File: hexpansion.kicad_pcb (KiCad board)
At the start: 2 copper layers, 32 x 36.6 mm, 7 parts, among them J1 Hexpansion-Connector, J2 Conn_02x10_Odd_Even

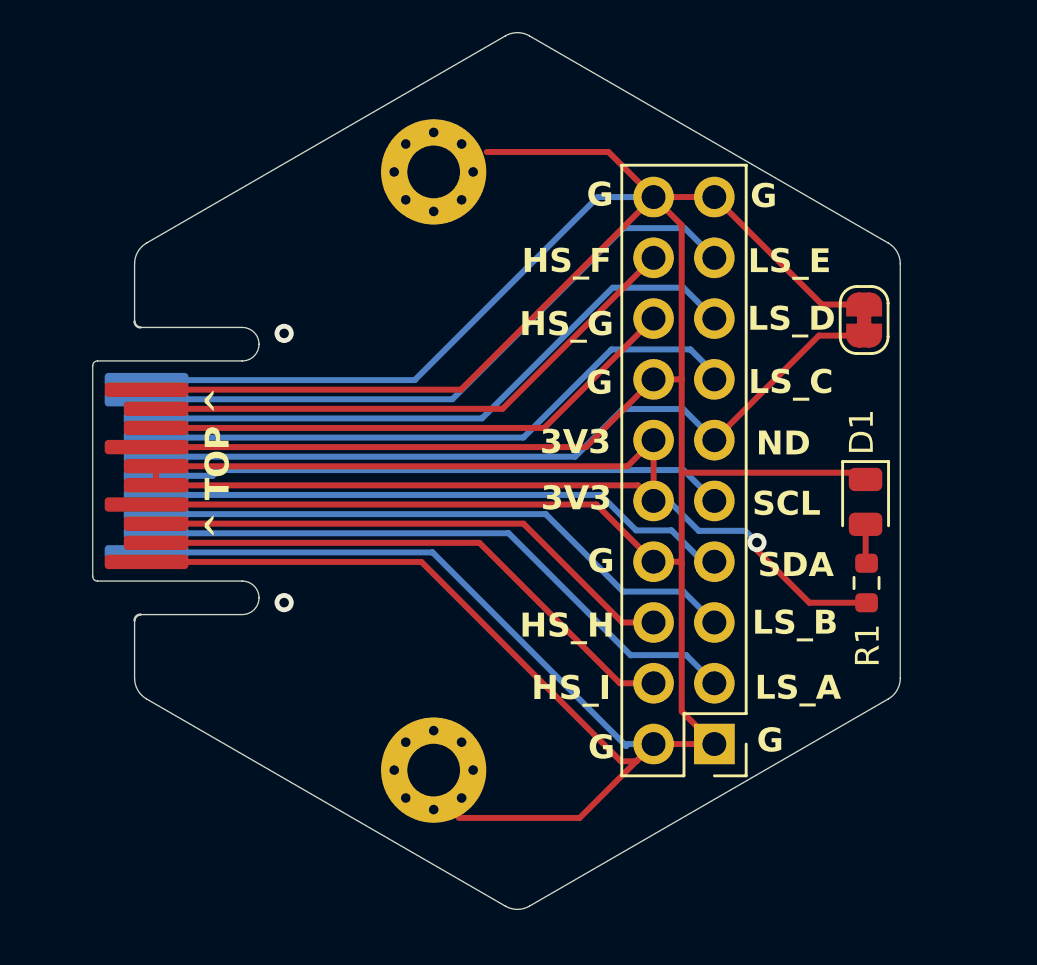
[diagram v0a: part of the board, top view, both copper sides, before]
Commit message: rough place of pcb
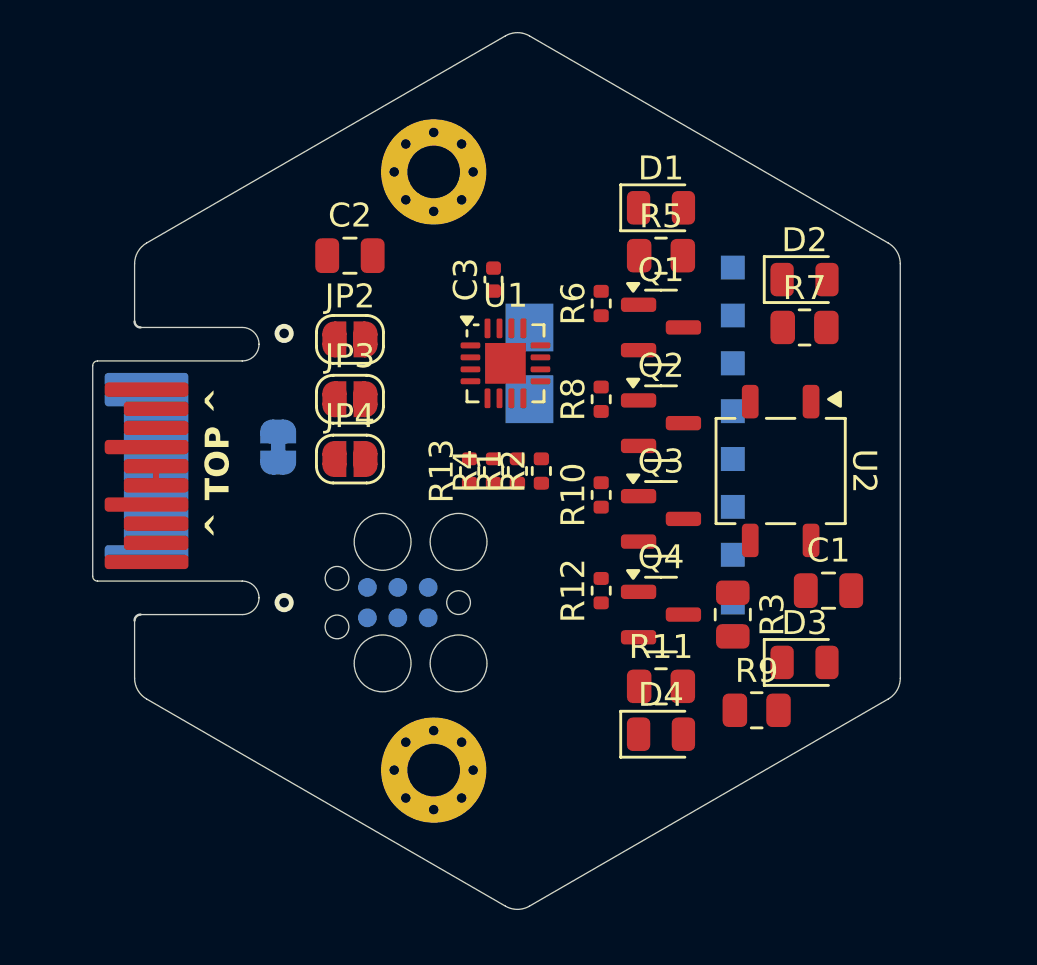
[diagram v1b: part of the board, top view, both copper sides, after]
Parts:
- added C1: 4.7 uF, Capacitor_SMD:C_0805_2012Metric, F.Cu at (129.0, 105.0)
- added C2: 4.7 uF, Capacitor_SMD:C_0805_2012Metric, F.Cu at (109.0, 91.0)
- added C3: 0.1 uF, Capacitor_SMD:C_0402_1005Metric, F.Cu at (115.0, 92.0)
- added D2: IR17-21C/TR8, LED_SMD:LED_0805_2012Metric, F.Cu at (128.0, 92.0)
- added D3: IR17-21C/TR8, LED_SMD:LED_0805_2012Metric, F.Cu at (128.0, 108.0)
- added D4: IR17-21C/TR8, LED_SMD:LED_0805_2012Metric, F.Cu at (122.0, 111.0)
- added JP2: SolderJumper_2_Open, Jumper:SolderJumper-2_P1.3mm_Open_RoundedPad1.0x1.5mm, F.Cu at (109.0, 94.5)
- added JP3: SolderJumper_2_Open, Jumper:SolderJumper-2_P1.3mm_Open_RoundedPad1.0x1.5mm, F.Cu at (109.0, 97.0)
- added JP4: SolderJumper_2_Open, Jumper:SolderJumper-2_P1.3mm_Open_RoundedPad1.0x1.5mm, F.Cu at (109.0, 99.5)
- added Q1: 2N7002, Package_TO_SOT_SMD:SOT-23, F.Cu at (122.0, 94.0)
- added Q2: 2N7002, Package_TO_SOT_SMD:SOT-23, F.Cu at (122.0, 98.0)
- added Q3: 2N7002, Package_TO_SOT_SMD:SOT-23, F.Cu at (122.0, 102.0)
- added Q4: 2N7002, Package_TO_SOT_SMD:SOT-23, F.Cu at (122.0, 106.0)
- added R10: 1k, Resistor_SMD:R_0402_1005Metric, F.Cu at (119.5, 101.0)
- added R11: 100, Resistor_SMD:R_0805_2012Metric, F.Cu at (122.0, 109.0)
- added R12: 1k, Resistor_SMD:R_0402_1005Metric, F.Cu at (119.5, 105.0)
- added R13: DNL, Resistor_SMD:R_0402_1005Metric, F.Cu at (114.0, 100.0)
- added R2: 10k, Resistor_SMD:R_0402_1005Metric, F.Cu at (117.0, 100.0)
- added R3: 100, Resistor_SMD:R_0805_2012Metric, F.Cu at (125.0, 106.0)
- added R4: 10k, Resistor_SMD:R_0402_1005Metric, F.Cu at (115.0, 100.0)
- added R5: 100, Resistor_SMD:R_0805_2012Metric, F.Cu at (122.0, 91.0)
- added R6: 1k, Resistor_SMD:R_0402_1005Metric, F.Cu at (119.5, 93.0)
- added R7: 100, Resistor_SMD:R_0805_2012Metric, F.Cu at (128.0, 94.0)
- added R8: 1k, Resistor_SMD:R_0402_1005Metric, F.Cu at (119.5, 97.0)
- added R9: 100, Resistor_SMD:R_0805_2012Metric, F.Cu at (126.0, 110.0)
- added TP1: TestPoint, TestPoint:TestPoint_Pad_2.0x2.0mm, B.Cu at (116.5, 94.0)
- added TP10: TestPoint_Small, TestPoint:TestPoint_Pad_1.0x1.0mm, B.Cu at (125.0, 101.5)
- added TP2: TestPoint, TestPoint:TestPoint_Pad_2.0x2.0mm, B.Cu at (116.5, 97.0)
- added TP3: TestPoint_Small, TestPoint:TestPoint_Pad_1.0x1.0mm, B.Cu at (125.0, 95.5)
- added TP4: TestPoint_Small, TestPoint:TestPoint_Pad_1.0x1.0mm, B.Cu at (125.0, 105.5)
- added TP5: TestPoint_Small, TestPoint:TestPoint_Pad_1.0x1.0mm, B.Cu at (125.0, 97.5)
- added TP6: TestPoint_Small, TestPoint:TestPoint_Pad_1.0x1.0mm, B.Cu at (125.0, 93.5)
- added TP7: TestPoint_Small, TestPoint:TestPoint_Pad_1.0x1.0mm, B.Cu at (125.0, 91.5)
- added TP8: TestPoint_Small, TestPoint:TestPoint_Pad_1.0x1.0mm, B.Cu at (125.0, 99.5)
- added TP9: TestPoint_Small, TestPoint:TestPoint_Pad_1.0x1.0mm, B.Cu at (125.0, 103.5)
- added U1: ~, Package_DFN_QFN:QFN-16-1EP_3x3mm_P0.5mm_EP1.7x1.7mm, F.Cu at (115.5, 95.5)
- added U2: ~, parts:IRM-H6XXT, F.Cu at (127.0, 100.0)
- D1: value LED -> IR17-21C/TR8
- J2: value Conn_02x10_Odd_Even -> Conn_ARM_SWD_TagConnect_TC2030; footprint Connector_PinHeader_2.54mm:PinHeader_2x10_P2.54mm_Vertical -> Connector:Tag-Connect_TC2030-IDC-FP_2x03_P1.27mm_Vertical; moved to B.Cu
- JP1: moved to B.Cu
- R1: value R -> 10k; footprint Resistor_SMD:R_0603_1608Metric -> Resistor_SMD:R_0402_1005Metric
- moved JP1 25.1 mm to (106.0, 99.0)
- moved R1 15.3 mm to (116.0, 100.0)
- moved D1 15.0 mm to (122.0, 89.0), turned to 0 degrees
- moved J2 14.5 mm to (111.0, 105.5)
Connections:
- D1 pad 1: /GND -> Net-(D1-K)
- H1 pad 1: /GND -> GND
- H2 pad 1: /GND -> GND
- J1 pad 1: /GND -> GND
- J1 pad 10: /GND -> GND
- J1 pad 11: /GND -> GND
- J1 pad 14: /GND -> GND
- J1 pad 15: /3V3 -> +3.3V
- J1 pad 16: /3V3 -> +3.3V
- J1 pad 17: /GND -> GND
- J1 pad 19: /HS_I -> unconnected-(J1-HS_I-Pad19)
- J1 pad 2: /LS_A -> unconnected-(J1-LS_A-Pad2)
- J1 pad 20: /GND -> GND
- J1 pad 3: /LS_B -> unconnected-(J1-LS_B-Pad3)
- J1 pad 7: /LS_C -> unconnected-(J1-LS_C-Pad7)
- J1 pad 8: /LS_D -> unconnected-(J1-LS_D-Pad8)
- J1 pad 9: /LS_E -> unconnected-(J1-LS_E-Pad9)
- J2 pad 1: /GND -> +3.3V
- J2 pad 2: /GND -> /SWDIO
- J2 pad 3: /LS_A -> /~{RST}
- J2 pad 4: /HS_I -> /SWCLK
- J2 pad 5: /LS_B -> GND
- J2 pad 6: /HS_H -> unconnected-(J2-SWO-Pad6)
- JP1 pad 2: /GND -> GND
- R1 pad 1: /3V3 -> +3.3V
- R1 pad 2: Net-(D1-A) -> /SDA
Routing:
- net /GND: track 207.4 -> 0.00 mm, vias 2 -> 0
- net /3V3: track 56.5 -> 0.00 mm, vias 1 -> 0
- net /HEXP_DET: track 32.8 -> 0.00 mm
- net /LS_E: track 27.2 -> 0.00 mm
- net /LS_D: track 26.1 -> 0.00 mm
- net /LS_A: track 25.9 -> 0.00 mm
- net /LS_C: track 25.5 -> 0.00 mm
- net /LS_B: track 25.2 -> 0.00 mm
- net /SDA: track 24.5 -> 0.00 mm
- net /SCL: track 24.0 -> 0.00 mm
- net /HS_F: track 23.4 -> 0.00 mm
- net /HS_I: track 23.2 -> 0.00 mm
- net /HS_G: track 22.7 -> 0.00 mm
- net /HS_H: track 22.5 -> 0.00 mm
- net Net-(D1-A): track 1.64 -> 0.00 mm
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- added copper zone on B.Cu, net GND
- added copper zone on F.Cu, net GND
- removed copper zone on B.Cu, net /GND
- removed copper zone on F.Cu, net /GND
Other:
- board text removed: "3V3"
- board text removed: "G"
- board text removed: "HS_F"
- board text removed: "HS_G"
- board text removed: "HS_H"
- board text removed: "HS_I"
- board text removed: "LS_A"
- board text removed: "LS_B"
- board text removed: "LS_C"
- board text removed: "LS_D"
- board text removed: "LS_E"
- board text removed: "ND"
- board text removed: "SCL"
- board text removed: "SDA"
